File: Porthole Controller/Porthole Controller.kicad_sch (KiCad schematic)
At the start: 19 parts, among them J1 STRIP1, J2 STRIP2, J3 STRIP3, J4 STRIP4, J5 INMP441, J6 Conn_02x04_Top_Bottom, J7 - +, J8 Conn_01x04, U1 113991054, U2 SN74AHCT125DR

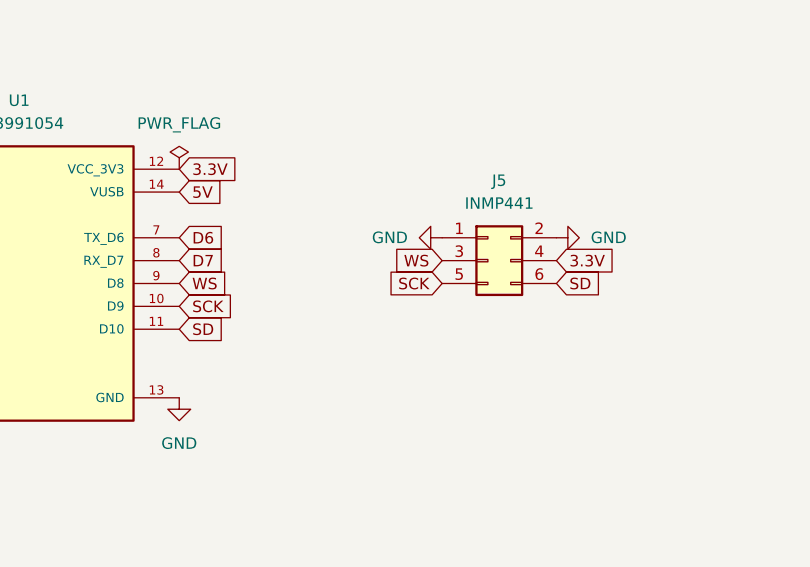
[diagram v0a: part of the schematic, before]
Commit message: Updated footprints
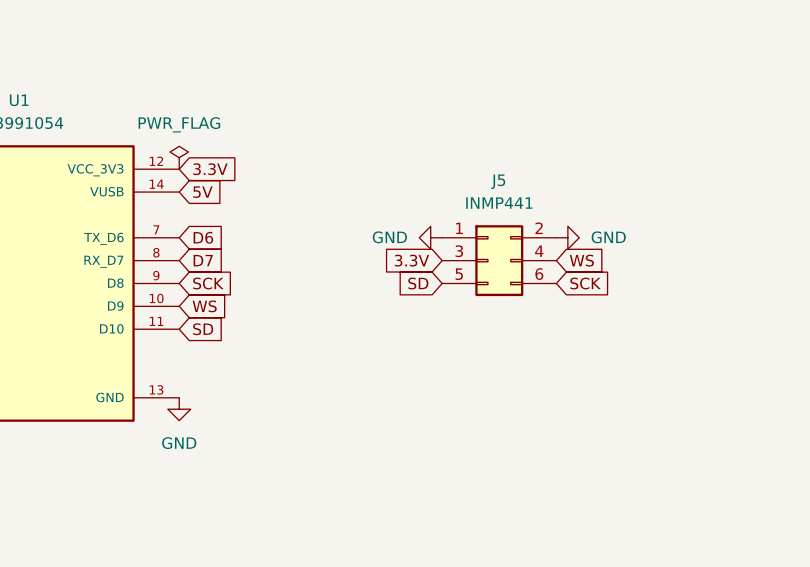
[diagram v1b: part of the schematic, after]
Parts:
- C2, C3, C4, C5: footprint Capacitor_THT:CP_Radial_D6.3mm_P2.50mm -> Capacitor_THT:CP_Radial_D8.0mm_P3.80mm
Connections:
- net 3.3V: now also J5.3 (Pin_3); no longer J5.4 (Pin_4)
- net SCK: now also J5.6 (Pin_6), U1.9 (D8); no longer J5.5 (Pin_5), U1.10 (D9)
- net SD: now also J5.5 (Pin_5); no longer J5.6 (Pin_6)
- net WS: now also J5.4 (Pin_4), U1.10 (D9); no longer J5.3 (Pin_3), U1.9 (D8)
